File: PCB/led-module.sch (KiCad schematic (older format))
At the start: 10 parts, among them J3 CONN_PWR, U1 TLC5940NT, U2 TLC5940NT

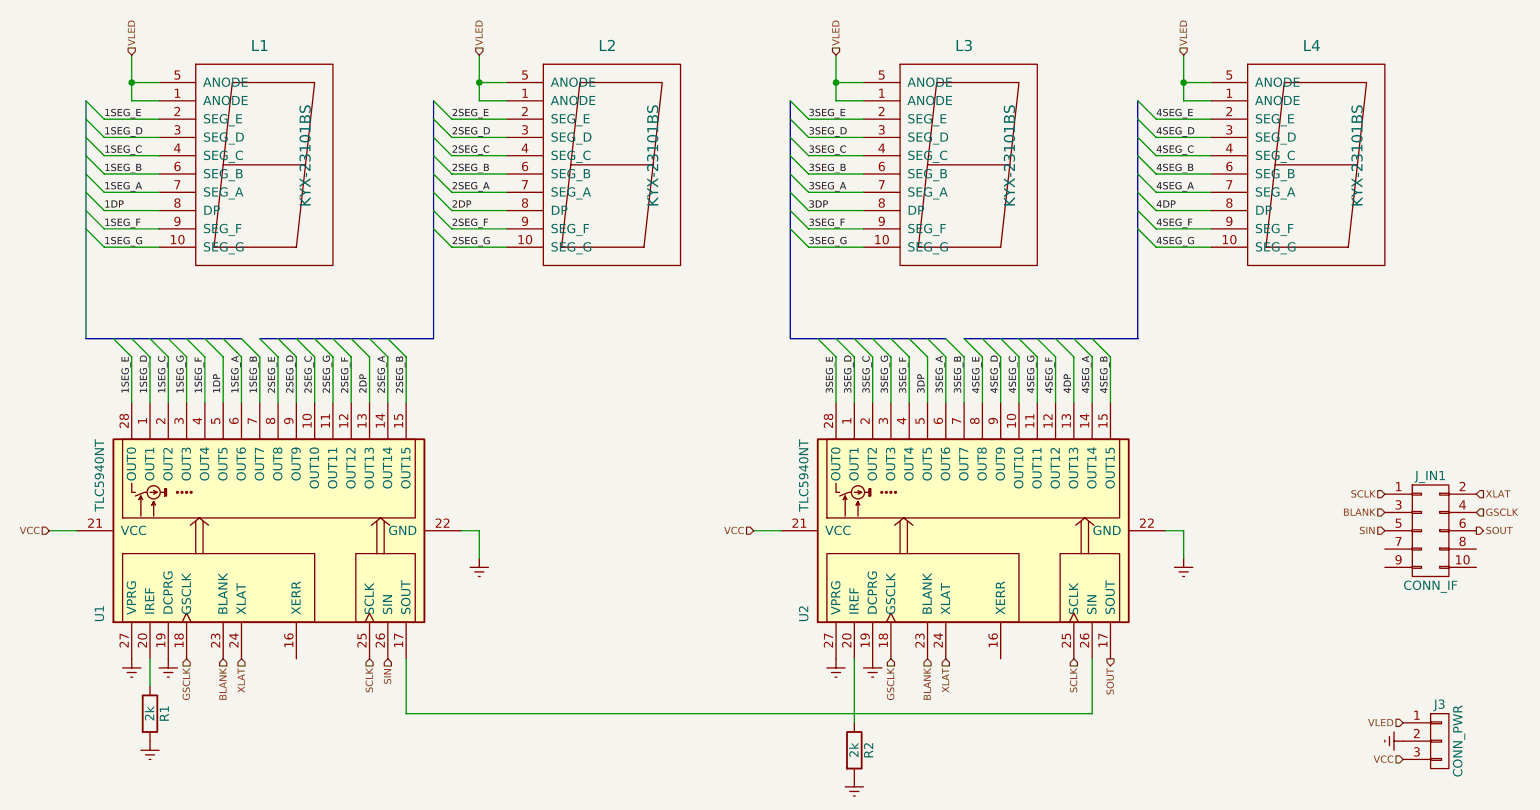
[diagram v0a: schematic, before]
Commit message: layoyt changed
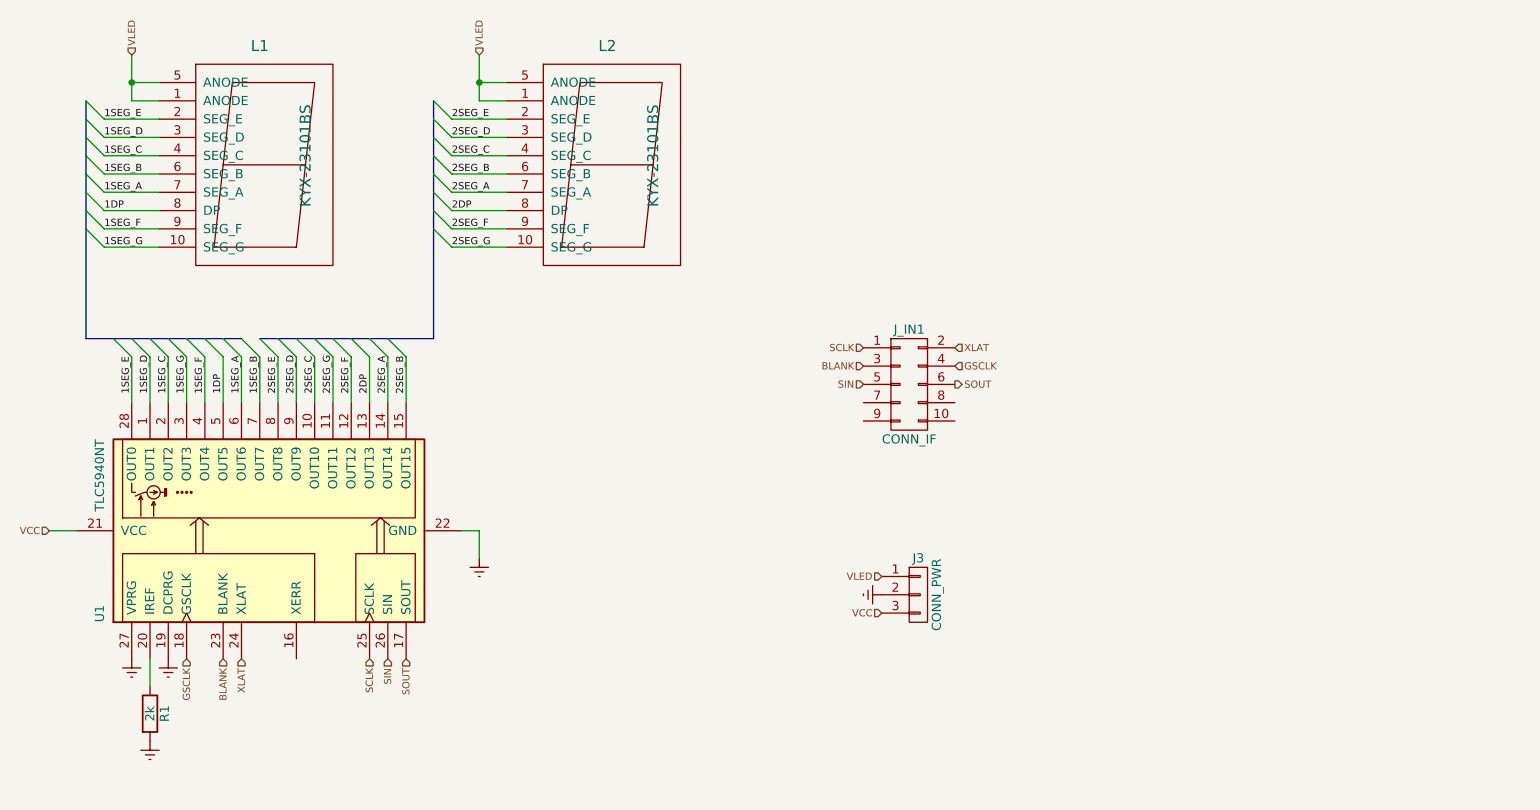
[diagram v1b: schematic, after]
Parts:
- removed L3, L4: KYX-23101BS, footprint:KYX-23101BS, symbol KYX-23101BS
- removed R2: 2k, Resistors_THT:R_Axial_DIN0207_L6.3mm_D2.5mm_P10.16mm_Horizontal, symbol R
- removed U2: TLC5940NT, Housings_DIP:DIP-28_W7.62mm, symbol TLC5940NT
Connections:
- net SOUT: now also U1.17 (SOUT)
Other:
- moved on the sheet: J3, J_IN1
